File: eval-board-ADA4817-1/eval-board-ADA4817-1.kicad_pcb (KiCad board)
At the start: 2 copper layers, 58.4 x 37.5 mm, 36 parts, among them U1 ADA4817-1

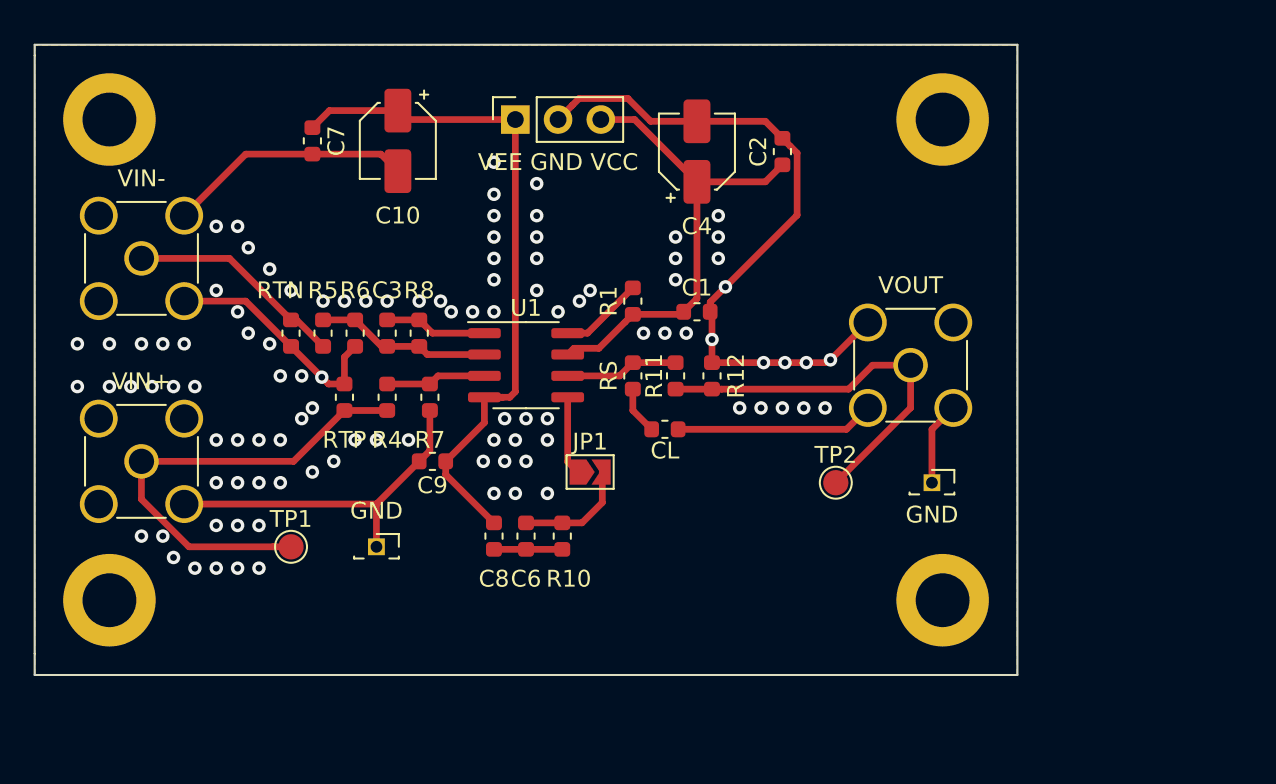
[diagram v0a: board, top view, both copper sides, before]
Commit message: updated
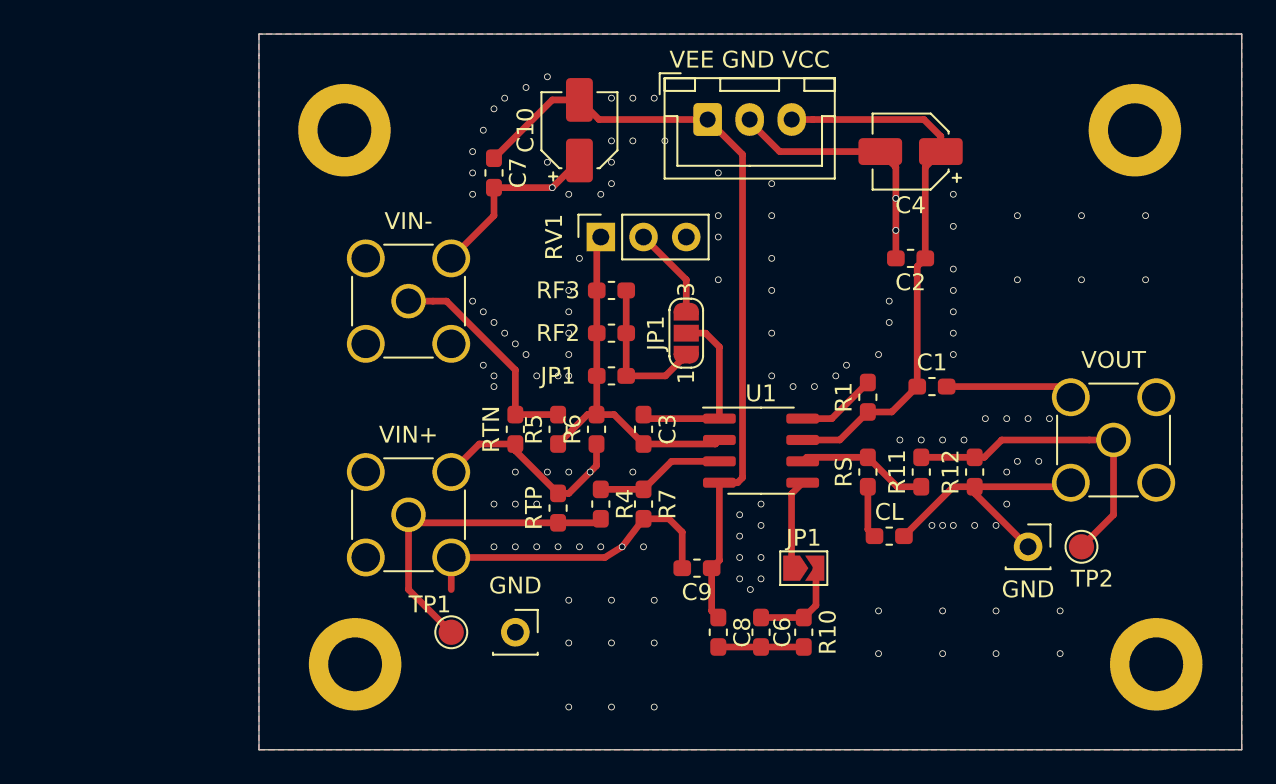
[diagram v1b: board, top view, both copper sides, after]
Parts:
- removed the CL at (140.3, 121.9)
- removed the GND at (156.2, 125.1)
- removed the GND at (123.2, 128.9)
- removed the JP1 at (135.9, 124.5)
- removed R8: RF, Resistor_SMD:R_0603_1608Metric
- removed the REF** at (107.3, 132.1)
- removed the REF** at (156.8, 132.1)
- removed the REF** at (156.8, 103.5)
- removed the REF** at (107.3, 103.5)
- removed the RS at (138.4, 118.7)
- removed the RTN at (118.1, 116.2)
- removed the RTP at (121.3, 120.0)
- removed the VEE GND VCC at (131.4, 103.5)
- added CL: CL, Capacitor_SMD:C_0603_1608Metric_Pad1.05x0.95mm_HandSolder, F.Cu at (153.7, 128.3)
- added GND: PinSocket_1x01_P2.54mm_Vertical, Connector_PinSocket_2.54mm:PinSocket_1x01_P2.54mm_Vertical, F.Cu at (131.4, 134.0)
- added GND: PinSocket_1x01_P2.54mm_Vertical, Connector_PinSocket_2.54mm:PinSocket_1x01_P2.54mm_Vertical, F.Cu at (161.9, 128.9)
- added JP1: SolderJumper-2_P1.3mm_Open_TrianglePad1.0x1.5mm, Jumper:SolderJumper-2_P1.3mm_Open_TrianglePad1.0x1.5mm, F.Cu at (148.6, 130.2)
- added JP1: Jumper_3_Open, Jumper:SolderJumper-3_P1.3mm_Open_RoundedPad1.0x1.5mm_NumberLabels, F.Cu at (141.6, 116.2)
- added JP1: R, Resistor_SMD:R_0603_1608Metric_Pad1.05x0.95mm_HandSolder, F.Cu at (137.2, 118.7)
- added REF**: MountingHole_3.2mm_M3_ISO14580_Pad, MountingHole:MountingHole_3.2mm_M3_ISO14580_Pad, F.Cu at (168.3, 104.1)
- added REF**: MountingHole_3.2mm_M3_ISO14580_Pad, MountingHole:MountingHole_3.2mm_M3_ISO14580_Pad, F.Cu at (169.5, 135.9)
- added REF**: MountingHole_3.2mm_M3_ISO14580_Pad, MountingHole:MountingHole_3.2mm_M3_ISO14580_Pad, F.Cu at (121.9, 135.9)
- added REF**: MountingHole_3.2mm_M3_ISO14580_Pad, MountingHole:MountingHole_3.2mm_M3_ISO14580_Pad, F.Cu at (121.3, 104.1)
- added RF2: R, Resistor_SMD:R_0603_1608Metric_Pad1.05x0.95mm_HandSolder, F.Cu at (137.2, 116.2)
- added RF3: R, Resistor_SMD:R_0603_1608Metric_Pad1.05x0.95mm_HandSolder, F.Cu at (137.2, 113.7)
- added RS: RS, Resistor_SMD:R_0603_1608Metric_Pad1.05x0.95mm_HandSolder, F.Cu at (152.4, 124.5)
- added RTN: RTN, Resistor_SMD:R_0603_1608Metric_Pad1.05x0.95mm_HandSolder, F.Cu at (131.4, 121.9)
- added RTP: RTP, Resistor_SMD:R_0603_1608Metric_Pad1.05x0.95mm_HandSolder, F.Cu at (134.0, 126.6)
- added RV1: R_POT, Connector_PinSocket_2.54mm:PinSocket_1x03_P2.54mm_Vertical, F.Cu at (136.5, 110.5)
- added VEE GND VCC: Conn_01x03_Male, Connector_JST:JST_XH_B3B-XH-A_1x03_P2.50mm_Vertical, F.Cu at (142.9, 103.5)
- C1, C2, C3, C6, C7, C8, C9: footprint Capacitor_SMD:C_0603_1608Metric -> Capacitor_SMD:C_0603_1608Metric_Pad1.05x0.95mm_HandSolder
- C10, C4: footprint Capacitor_SMD:CP_Elec_4x5.3 -> Capacitor_SMD:CP_Elec_4x5.4
- R1, R10, R11, R12, R4, R5, R6, R7: footprint Resistor_SMD:R_0603_1608Metric -> Resistor_SMD:R_0603_1608Metric_Pad1.05x0.95mm_HandSolder
- moved R10 17.5 mm to (148.6, 134.0)
- moved C9 17.0 mm to (142.2, 130.2)
- moved R12 16.6 mm to (158.8, 124.5), turned to 90 degrees
- moved C3 16.3 mm to (139.1, 121.9)
- moved VIN+ 16.2 mm to (125.1, 127.0)
- moved VIN- 16.1 mm to (125.1, 114.3)
- moved R11 15.7 mm to (155.6, 124.5), turned to 90 degrees
- moved R6 15.4 mm to (136.3, 121.9)
- moved R5 15.1 mm to (134.0, 121.9), turned to 90 degrees
- moved R1 15.1 mm to (152.4, 120.0)
- moved TP2 15.1 mm to (165.1, 128.9)
- moved U1 14.9 mm to (146.1, 123.2)
- moved C1 14.7 mm to (156.2, 119.4)
- moved C8 14.5 mm to (143.5, 134.0)
- moved R4 14.2 mm to (136.5, 126.4)
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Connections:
- C10 pad 1: /VEE -> GNDREF
- C10 pad 2: GNDREF -> /VEE
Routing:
- net GNDREF: track 107.3 -> 82.0 mm, vias 103 -> 127
- net Net-(C3-Pad2): track 10.4 -> 21.8 mm
- net Net-(JP1-Pad1): track 0.00 -> 9.16 mm
- net Net-(J3-Pad1): track 28.2 -> 19.8 mm
- net /VEE: track 40.5 -> 46.6 mm
- net Net-(JP1-Pad3): track 0.00 -> 5.47 mm
- net Net-(C3-Pad1): track 6.11 -> 11.2 mm
- net Net-(J5-Pad1): track 23.4 -> 19.0 mm
- net /VCC: track 28.7 -> 32.9 mm
- net Net-(R4-Pad1): track 5.98 -> 7.74 mm
- net Net-(R11-Pad1): track 6.74 -> 7.87 mm
- net Net-(C6-Pad1): track 4.06 -> 5.08 mm
- net Net-(C6-Pad2): track 11.7 -> 11.1 mm
- net (no net): vias 0 -> 1
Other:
- board size 58.4 x 37.5 mm -> 58.4 x 42.5 mm
